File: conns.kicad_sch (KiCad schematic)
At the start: 5 parts, among them J1 GSB1C4621DS1HR

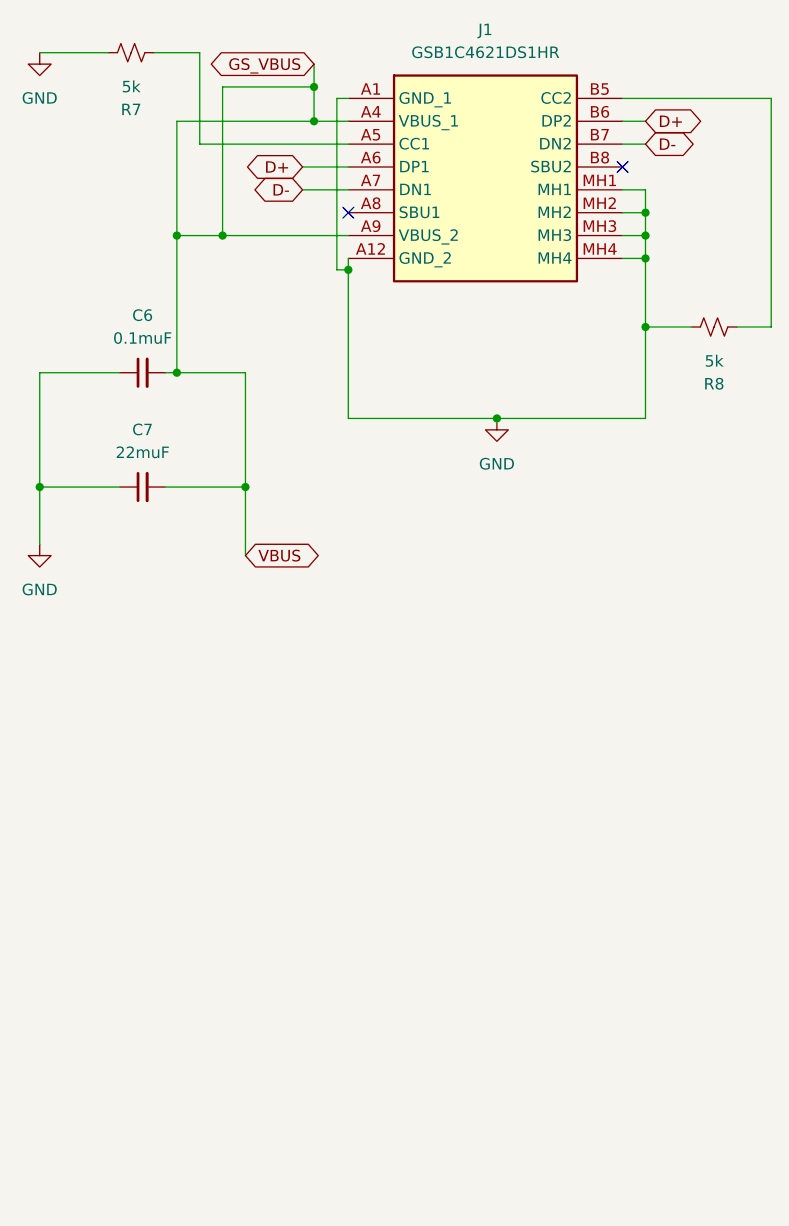
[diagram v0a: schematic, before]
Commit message: finishing mcu design schematic
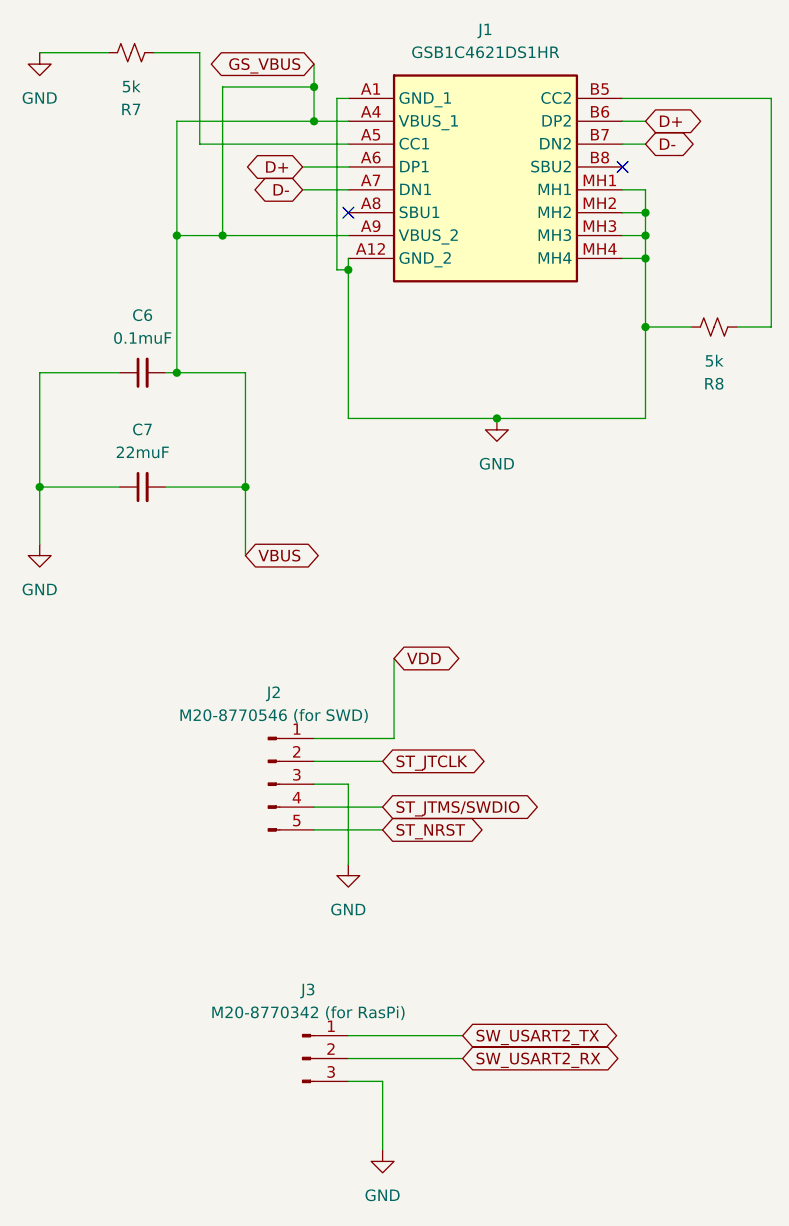
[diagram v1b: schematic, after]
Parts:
- added J2: M20-8770546 (for SWD), Connector_PinSocket_2.54mm:PinSocket_1x05_P2.54mm_Vertical, symbol Connector:Conn_01x05_Pin
- added J3: M20-8770342 (for RasPi), Connector_PinSocket_2.54mm:PinSocket_1x03_P2.54mm_Vertical, symbol Connector:Conn_01x03_Pin
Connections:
- net GND: now also J2.3 (Pin_3), J3.3 (Pin_3)
- new net ST_JTCLK: J2.2 (Pin_2)
- new net ST_JTMS/SWDIO: J2.4 (Pin_4)
- new net ST_NRST: J2.5 (Pin_5)
- new net SW_USART2_RX: J3.2 (Pin_2)
- new net SW_USART2_TX: J3.1 (Pin_1)
- new net VDD: J2.1 (Pin_1)
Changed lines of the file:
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@@
+    (stroke (width 0) (type default))
+  )
+  (wire (pts (xy 59.69 142.24) (xy 72.39 142.24))
     (stroke (width 0) (type default))
   )
@@
     (stroke (width 0) (type default))
   )
+  (wire (pts (xy 59.69 144.78) (xy 63.5 144.78))
+    (stroke (width 0) (type default))
+  )
   (wire (pts (xy 92.71 45.72) (xy 92.71 48.26))
     (stroke (width 0) (type default))
@@
     (stroke (width 0) (type default))
   )
+  (wire (pts (xy 64.77 106.68) (xy 64.77 97.79))
+    (stroke (width 0) (type default))
+  )
+  (wire (pts (xy 55.88 114.3) (xy 63.5 114.3))
+    (stroke (width 0) (type default))
+  )
   (wire (pts (xy 54.61 45.72) (xy 59.69 45.72))
     (stroke (width 0) (type default))
@@
     (stroke (width 0) (type default))
   )
+  (wire (pts (xy 55.88 116.84) (xy 63.5 116.84))
+    (stroke (width 0) (type default))
+  )
   (wire (pts (xy 25.4 66.04) (xy 34.29 66.04))
     (stroke (width 0) (type default))
@@
     (stroke (width 0) (type default))
   )
+  (wire (pts (xy 59.69 139.7) (xy 72.39 139.7))
+    (stroke (width 0) (type default))
+  )
   (wire (pts (xy 58.42 35.56) (xy 58.42 54.61))
     (stroke (width 0) (type default))
@@
     (stroke (width 0) (type default))
   )
+  (wire (pts (xy 55.88 109.22) (xy 63.5 109.22))
+    (stroke (width 0) (type default))
+  )
+  (wire (pts (xy 55.88 111.76) (xy 59.69 111.76))
+    (stroke (width 0) (type default))
+  )
   (wire (pts (xy 40.64 38.1) (xy 55.88 38.1))
     (stroke (width 0) (type default))
@@
     (stroke (width 0) (type default))
   )
+  (wire (pts (xy 59.69 111.76) (xy 59.69 120.65))
+    (stroke (width 0) (type default))
+  )
+  (wire (pts (xy 55.88 106.68) (xy 64.77 106.68))
+    (stroke (width 0) (type default))
+  )
   (wire (pts (xy 40.64 50.8) (xy 40.64 66.04))
     (stroke (width 0) (type default))
@@
   (wire (pts (xy 92.71 48.26) (xy 92.71 50.8))
     (stroke (width 0) (type default))
+  )
+  (wire (pts (xy 63.5 144.78) (xy 63.5 152.4))
+    (stroke (width 0) (type default))
+  )
+  (global_label "ST_JTMS{slash}SWDIO" (shape bidirectional) (at 63.5 114.3 0) (fields_autoplaced)
+    (effects (font (size 1.27 1.27)) (justify left))
+    (property "Intersheetrefs" "${INTERSHEET_REFS}" (at 82.534 114.3 0)
+      (effects (font (size 1.27 1.27)) (justify left) hide)
+    )
   )
   (global_label "GS_VBUS" (shape bidirectional) (at 55.88 31.75 180) (fields_autoplaced)
@@
     )
   )
+  (global_label "VDD" (shape bidirectional) (at 64.77 97.79 0) (fields_autoplaced)
+    (effects (font (size 1.27 1.27)) (justify left))
+    (property "Intersheetrefs" "${INTERSHEET_REFS}" (at 72.4951 97.79 0)
+      (effects (font (size 1.27 1.27)) (justify left) hide)
+    )
+  )
+  (global_label "SW_USART2_TX" (shape bidirectional) (at 72.39 139.7 0) (fields_autoplaced)
+    (effects (font (size 1.27 1.27)) (justify left))
+    (property "Intersheetrefs" "${INTERSHEET_REFS}" (at 90.3354 139.7 0)
+      (effects (font (size 1.27 1.27)) (justify left) hide)
+    )
+  )
   (global_label "D+" (shape bidirectional) (at 54.61 43.18 180) (fields_autoplaced)
     (effects (font (size 1.27 1.27)) (justify right))
@@
     )
   )
+  (global_label "ST_NRST" (shape bidirectional) (at 63.5 116.84 0) (fields_autoplaced)
+    (effects (font (size 1.27 1.27)) (justify left))
+    (property "Intersheetrefs" "${INTERSHEET_REFS}" (at 75.5188 116.84 0)
+      (effects (font (size 1.27 1.27)) (justify left) hide)
+    )
+  )
+  (global_label "SW_USART2_RX" (shape bidirectional) (at 72.39 142.24 0) (fields_autoplaced)
+    (effects (font (size 1.27 1.27)) (justify left))
+    (property "Intersheetrefs" "${INTERSHEET_REFS}" (at 90.6378 142.24 0)
+      (effects (font (size 1.27 1.27)) (justify left) hide)
+    )
+  )
+  (global_label "ST_JTCLK" (shape bidirectional) (at 63.5 109.22 0) (fields_autoplaced)
+    (effects (font (size 1.27 1.27)) (justify left))
+    (property "Intersheetrefs" "${INTERSHEET_REFS}" (at 76.2445 109.22 0)
+      (effects (font (size 1.27 1.27)) (justify left) hide)
+    )
+  )
   (global_label "D-" (shape bidirectional) (at 92.71 40.64 0) (fields_autoplaced)
     (effects (font (size 1.27 1.27)) (justify left))
@@
     )
   )
+  (symbol (lib_id "power:GND") (at 63.5 152.4 0) (unit 1)
+    (in_bom yes) (on_board yes) (dnp no) (fields_autoplaced)
+    (property "Reference" "#PWR056" (at 63.5 158.75 0)
+      (effects (font (size 1.27 1.27)) hide)
+    )
+    (property "Value" "GND" (at 63.5 157.48 0)
+      (effects (font (size 1.27 1.27)))
+    )
+    (property "Footprint" "" (at 63.5 152.4 0)
+      (effects (font (size 1.27 1.27)) hide)
+    )
+    (property "Datasheet" "" (at 63.5 152.4 0)
+      (effects (font (size 1.27 1.27)) hide)
+    )
+    (pin "1")
+    (instances
+      (project "radar2"
+        (path "/4b235fed-a05d-46ae-99fd-4a907d865754/dfc10a02-f047-425a-8f9d-e4a822e029f8"
+          (reference "#PWR056") (unit 1)
+        )
+      )
+    )
+  )
   (symbol (lib_id "Device:C_Small") (at 36.83 66.04 90) (unit 1)
     (in_bom yes) (on_board yes) (dnp no) (fields_autoplaced)
@@
         (path "/4b235fed-a05d-46ae-99fd-4a907d865754/dfc10a02-f047-425a-8f9d-e4a822e029f8"
           (reference "R8") (unit 1)
+        )
+      )
+    )
+  )
+  (symbol (lib_id "Connector:Conn_01x03_Pin") (at 54.61 142.24 0) (unit 1)
+    (in_bom yes) (on_board yes) (dnp no) (fields_autoplaced)
+    (property "Reference" "J3" (at 55.245 134.62 0)
+      (effects (font (size 1.27 1.27)))
+    )
+    (property "Value" "M20-8770342 (for RasPi)" (at 55.245 137.16 0)
+      (effects (font (size 1.27 1.27)))
+    )
+    (property "Footprint" "Connector_PinSocket_2.54mm:PinSocket_1x03_P2.54mm_Vertical" (at 54.61 142.24 0)
+      (effects (font (size 1.27 1.27)) hide)
+    )
+    (property "Datasheet" "~" (at 54.61 142.24 0)
+      (effects (font (size 1.27 1.27)) hide)
+    )
+    (pin "3")
+    (pin "1")
+    (pin "2")
+    (instances
+      (project "radar2"
+        (path "/4b235fed-a05d-46ae-99fd-4a907d865754/dfc10a02-f047-425a-8f9d-e4a822e029f8"
+          (reference "J3") (unit 1)
+        )
+      )
+    )
+  )
+  (symbol (lib_id "Connector:Conn_01x05_Pin") (at 50.8 111.76 0) (unit 1)
+    (in_bom yes) (on_board yes) (dnp no) (fields_autoplaced)
+    (property "Reference" "J2" (at 51.435 101.6 0)
+      (effects (font (size 1.27 1.27)))
+    )
+    (property "Value" "M20-8770546 (for SWD)" (at 51.435 104.14 0)
+      (effects (font (size 1.27 1.27)))
+    )
+    (property "Footprint" "Connector_PinSocket_2.54mm:PinSocket_1x05_P2.54mm_Vertical" (at 50.8 111.76 0)
+      (effects (font (size 1.27 1.27)) hide)
+    )
+    (property "Datasheet" "~" (at 50.8 111.76 0)
+      (effects (font (size 1.27 1.27)) hide)
+    )
+    (pin "4")
+    (pin "2")
+    (pin "5")
+    (pin "1")
+    (pin "3")
+    (instances
+      (project "radar2"
+        (path "/4b235fed-a05d-46ae-99fd-4a907d865754/dfc10a02-f047-425a-8f9d-e4a822e029f8"
+          (reference "J2") (unit 1)
         )
       )
@@
         )
       )
+    )
+  )
+  (symbol (lib_id "power:GND") (at 59.69 120.65 0) (unit 1)
+    (in_bom yes) (on_board yes) (dnp no) (fields_autoplaced)
+    (property "Reference" "#PWR053" (at 59.69 127 0)
+      (effects (font (size 1.27 1.27)) hide)
+    )
+    (property "Value" "GND" (at 59.69 125.73 0)
+      (effects (font (size 1.27 1.27)))
+    )
+    (property "Footprint" "" (at 59.69 120.65 0)
+      (effects (font (size 1.27 1.27)) hide)
+    )
+    (property "Datasheet" "" (at 59.69 120.65 0)
+      (effects (font (size 1.27 1.27)) hide)
+    )
+    (pin "1")
+    (instances
+      (project "radar2"
+        (path "/4b235fed-a05d-46ae-99fd-4a907d865754/dfc10a02-f047-425a-8f9d-e4a822e029f8"
+          (reference "#PWR053") (unit 1)
+        )
+      )
